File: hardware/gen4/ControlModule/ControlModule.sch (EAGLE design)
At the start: 16 parts, among them IC1 XMEGA16A4A

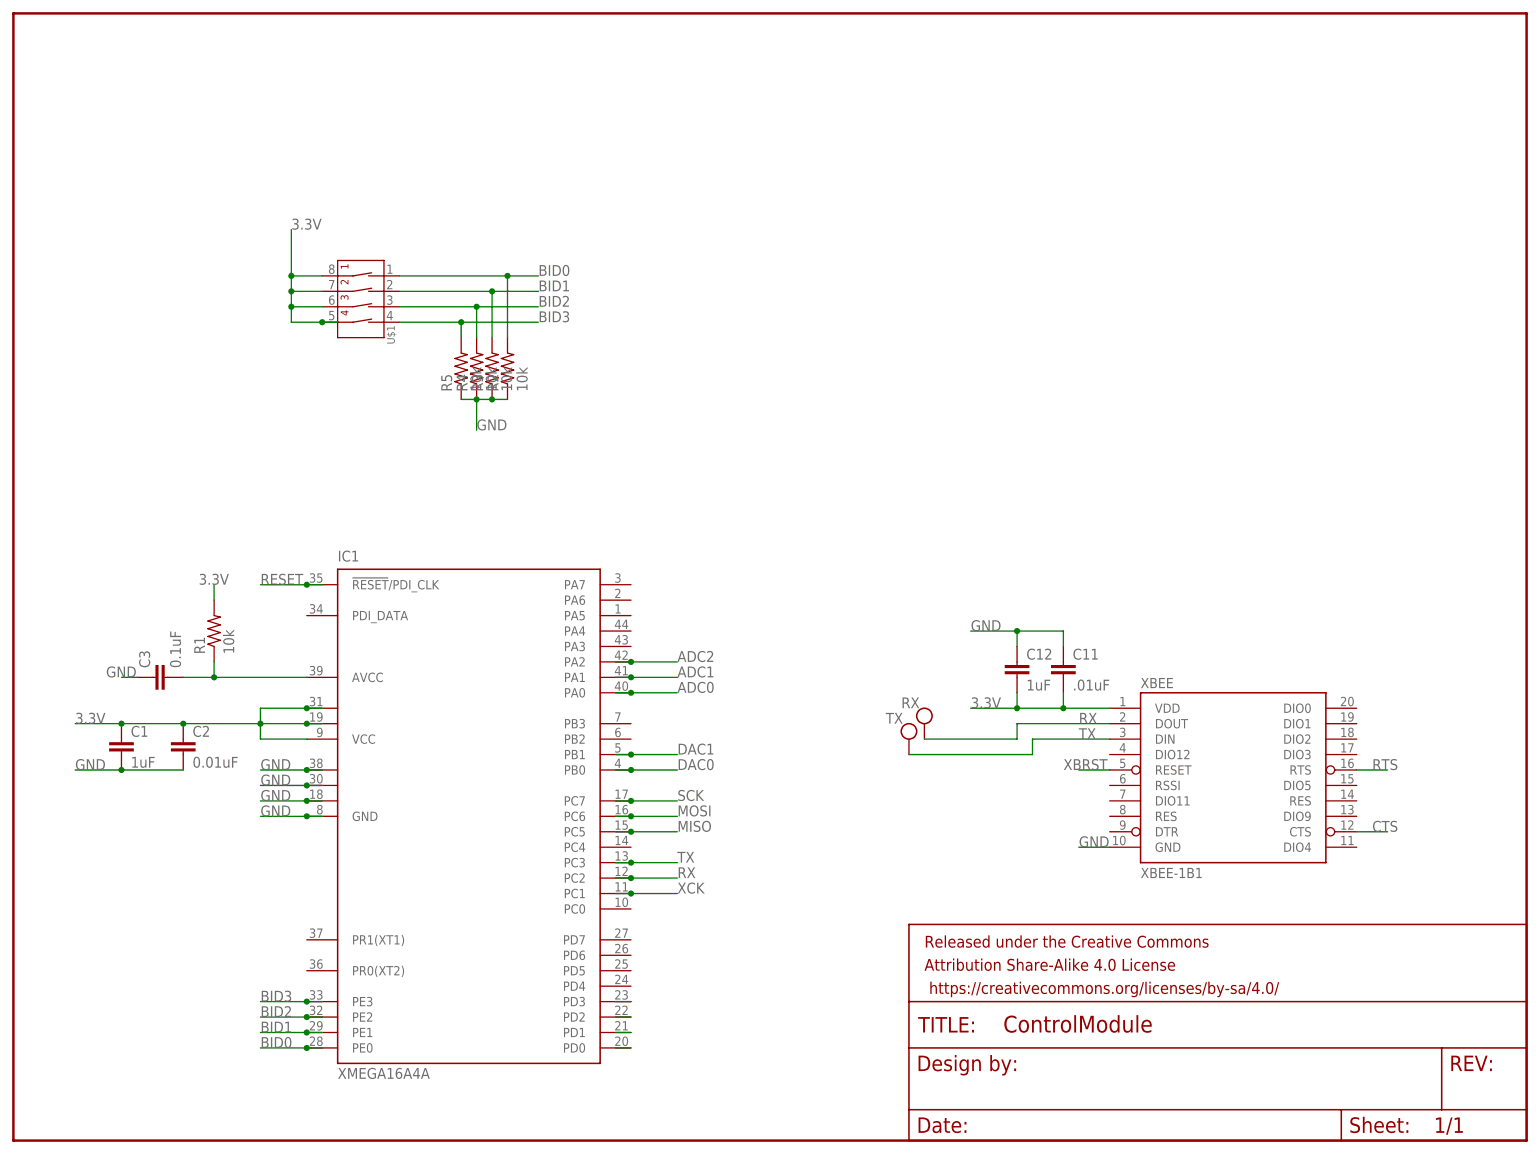
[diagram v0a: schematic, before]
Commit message: Working on xbee stuff for microboard
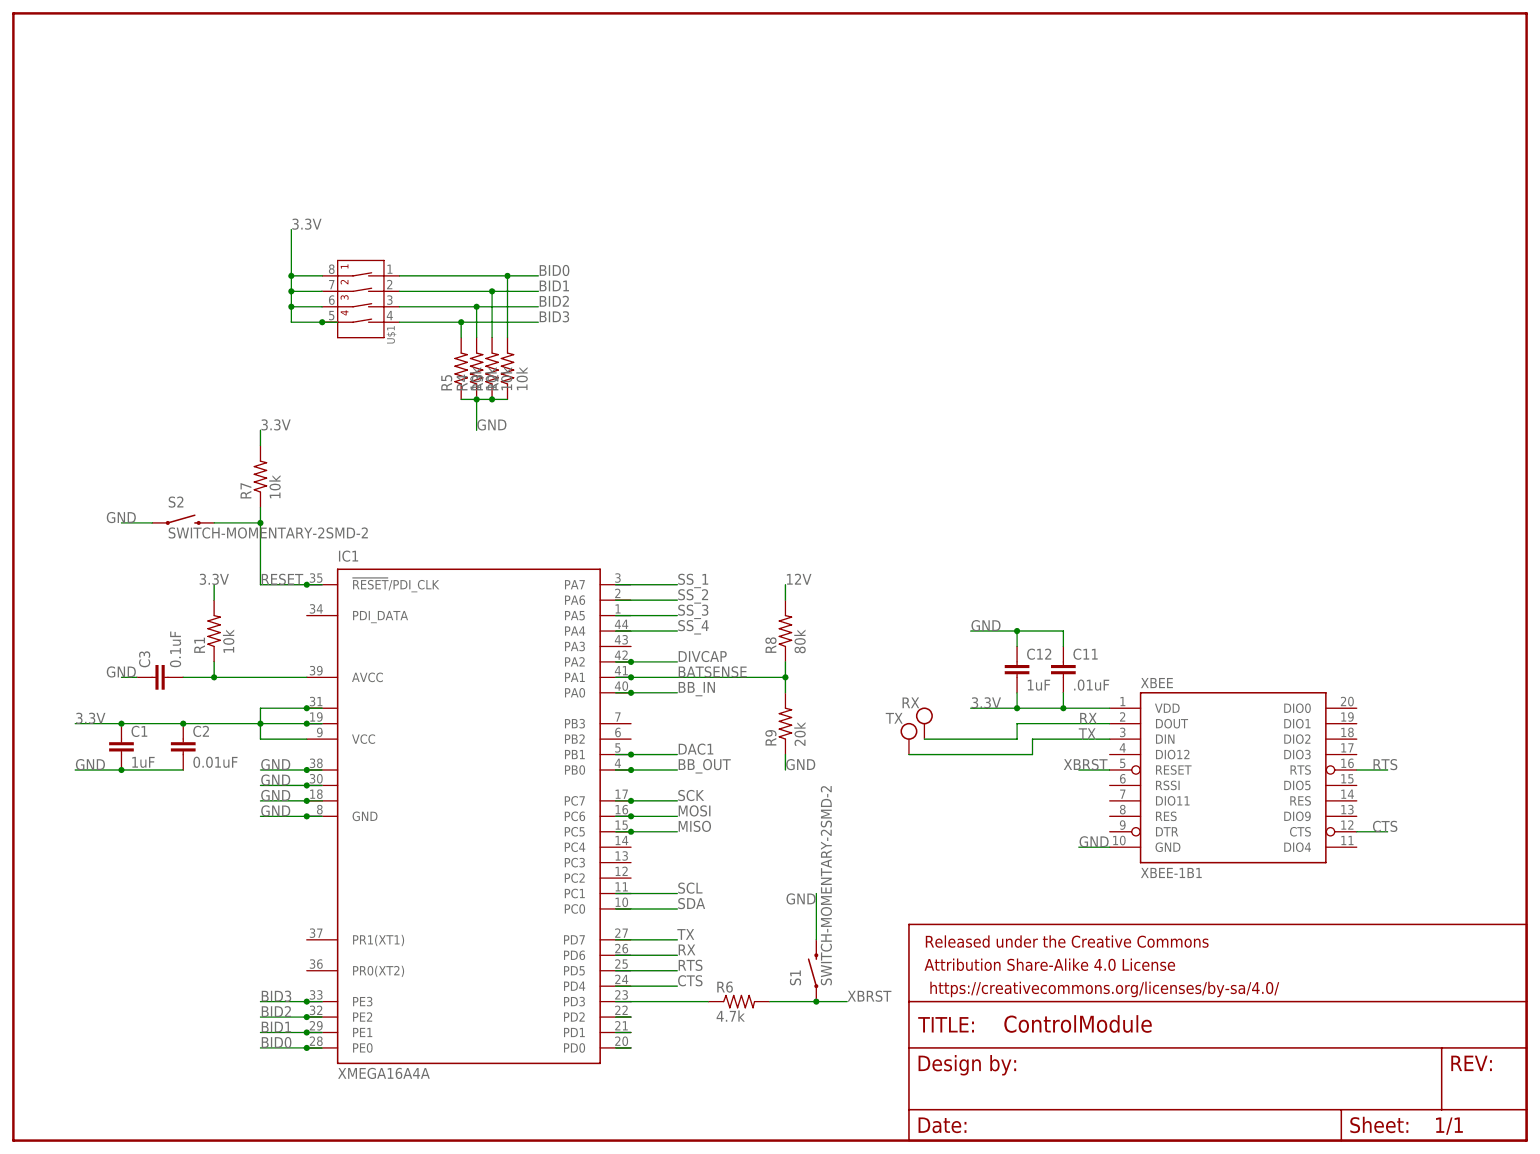
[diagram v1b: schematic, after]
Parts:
- added R6: 4.7k, SparkFun-Passives:RESISTOR0805-RES
- added R7: 10k, SparkFun-Passives:RESISTOR0805-RES
- added R8: 80k, SparkFun-Passives:RESISTOR0805-RES
- added R9: 20k, SparkFun-Passives:RESISTOR0805-RES
- added S1, S2: SWITCH-MOMENTARY-2SMD-2, SparkFun-Electromechanical:SWITCH-MOMENTARY-2SMD-2
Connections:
- net ADC0 renamed BB_IN
- net ADC2 renamed DIVCAP
- net DAC0 renamed BB_OUT
- removed net ADC1: IC1.PA1
- removed net XCK: IC1.PC1
- new net 12V: R8.2
- new net BATSENSE: IC1.PA1, R8.1, R9.2
- net 3.3V: now also R7.2
- net GND: now also R9.1, S1.2, S2.1
- net N$5: now also R6.1
- net RESET: now also R7.1, S2.2
- net RX: no longer IC1.PC2
- net TX: no longer IC1.PC3
- net XBRST: now also R6.2, S1.1
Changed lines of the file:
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@@
 <part name="RX" library="gen3" deviceset="TEST_PT" device=""/>
 <part name="TX" library="gen3" deviceset="TEST_PT" device=""/>
+<part name="R6" library="SparkFun-Passives" deviceset="RESISTOR" device="0805-RES" value="4.7k"/>
+<part name="S1" library="SparkFun-Electromechanical" deviceset="SWITCH-MOMENTARY-2" device="SMD-2"/>
+<part name="S2" library="SparkFun-Electromechanical" deviceset="SWITCH-MOMENTARY-2" device="SMD-2"/>
+<part name="R7" library="SparkFun-Passives" deviceset="RESISTOR" device="0805-RES" value="10k"/>
+<part name="R8" library="SparkFun-Passives" deviceset="RESISTOR" device="0805-RES" value="80k"/>
+<part name="R9" library="SparkFun-Passives" deviceset="RESISTOR" device="0805-RES" value="20k"/>
 </parts>
 <sheets>
@@
 <instance part="RX" gate="G$1" x="149.86" y="68.58"/>
 <instance part="TX" gate="G$1" x="147.32" y="66.04"/>
+<instance part="R6" gate="G$1" x="119.38" y="22.86"/>
+<instance part="S1" gate="G$1" x="132.08" y="27.94" rot="R90"/>
+<instance part="S2" gate="G$1" x="27.94" y="101.6"/>
+<instance part="R7" gate="G$1" x="40.64" y="109.22" rot="R90"/>
+<instance part="R8" gate="G$1" x="127" y="83.82" rot="R90"/>
+<instance part="R9" gate="G$1" x="127" y="68.58" rot="R90"/>
 </instances>
 <busses>
@@
 </net>
 <net name="TX" class="0">
-<segment>
-<wire x1="99.06" y1="45.72" x2="101.6" y2="45.72" width="0.1524" layer="91"/>
-<label x="109.22" y="45.72" size="1.778" layer="95"/>
-<pinref part="IC1" gate="G$1" pin="PC3"/>
-<wire x1="101.6" y1="45.72" x2="109.22" y2="45.72" width="0.1524" layer="91"/>
-<junction x="101.6" y="45.72"/>
-</segment>
 <segment>
 <pinref part="XBEE" gate="G$1" pin="DIN"/>
@@
 <wire x1="167.64" y1="66.04" x2="180.34" y2="66.04" width="0.1524" layer="91"/>
 </segment>
+<segment>
+<wire x1="99.06" y1="33.02" x2="109.22" y2="33.02" width="0.1524" layer="91"/>
+<label x="109.22" y="33.02" size="1.778" layer="95"/>
+</segment>
 </net>
 <net name="RX" class="0">
-<segment>
-<wire x1="99.06" y1="43.18" x2="101.6" y2="43.18" width="0.1524" layer="91"/>
-<label x="109.22" y="43.18" size="1.778" layer="95"/>
-<pinref part="IC1" gate="G$1" pin="PC2"/>
-<wire x1="101.6" y1="43.18" x2="109.22" y2="43.18" width="0.1524" layer="91"/>
-<junction x="101.6" y="43.18"/>
-</segment>
 <segment>
 <pinref part="XBEE" gate="G$1" pin="DOUT"/>
@@
 <wire x1="165.1" y1="66.04" x2="149.86" y2="66.04" width="0.1524" layer="91"/>
 </segment>
-</net>
-<net name="XCK" class="0">
-<segment>
-<wire x1="99.06" y1="40.64" x2="101.6" y2="40.64" width="0.1524" layer="91"/>
-<label x="109.22" y="40.64" size="1.778" layer="95"/>
-<pinref part="IC1" gate="G$1" pin="PC1"/>
-<wire x1="101.6" y1="40.64" x2="109.22" y2="40.64" width="0.1524" layer="91"/>
-<junction x="101.6" y="40.64"/>
-</segment>
-</net>
-<net name="ADC0" class="0">
+<segment>
+<wire x1="99.06" y1="30.48" x2="109.22" y2="30.48" width="0.1524" layer="91"/>
+<label x="109.22" y="30.48" size="1.778" layer="95"/>
+</segment>
+</net>
+<net name="BB_IN" class="0">
 <segment>
 <wire x1="99.06" y1="73.66" x2="101.6" y2="73.66" width="0.1524" layer="91"/>
@@
 </segment>
 </net>
-<net name="ADC1" class="0">
+<net name="BATSENSE" class="0">
 <segment>
 <wire x1="99.06" y1="76.2" x2="101.6" y2="76.2" width="0.1524" layer="91"/>
 <label x="109.22" y="76.2" size="1.778" layer="95"/>
 <pinref part="IC1" gate="G$1" pin="PA1"/>
-<wire x1="101.6" y1="76.2" x2="109.22" y2="76.2" width="0.1524" layer="91"/>
 <junction x="101.6" y="76.2"/>
-</segment>
-</net>
-<net name="ADC2" class="0">
+<wire x1="101.6" y1="76.2" x2="127" y2="76.2" width="0.1524" layer="91"/>
+<wire x1="127" y1="76.2" x2="127" y2="73.66" width="0.1524" layer="91"/>
+<wire x1="127" y1="76.2" x2="127" y2="78.74" width="0.1524" layer="91"/>
+<junction x="127" y="76.2"/>
+<pinref part="R8" gate="G$1" pin="1"/>
+<pinref part="R9" gate="G$1" pin="2"/>
+</segment>
+</net>
+<net name="DIVCAP" class="0">
 <segment>
 <wire x1="99.06" y1="78.74" x2="101.6" y2="78.74" width="0.1524" layer="91"/>
@@
 <wire x1="48.26" y1="91.44" x2="40.64" y2="91.44" width="0.1524" layer="91"/>
 <junction x="48.26" y="91.44"/>
+<wire x1="40.64" y1="91.44" x2="40.64" y2="101.6" width="0.1524" layer="91"/>
+<wire x1="40.64" y1="101.6" x2="40.64" y2="104.14" width="0.1524" layer="91"/>
+<wire x1="40.64" y1="101.6" x2="33.02" y2="101.6" width="0.1524" layer="91"/>
+<junction x="40.64" y="101.6"/>
+<pinref part="S2" gate="G$1" pin="2"/>
+<pinref part="R7" gate="G$1" pin="1"/>
 </segment>
 </net>
@@
 <junction x="165.1" y="83.82"/>
 <label x="157.48" y="83.82" size="1.778" layer="95"/>
+</segment>
+<segment>
+<pinref part="S1" gate="G$1" pin="2"/>
+<wire x1="132.08" y1="33.02" x2="132.08" y2="40.64" width="0.1524" layer="91"/>
+<label x="132.08" y="40.64" size="1.778" layer="95" rot="R180"/>
+</segment>
+<segment>
+<pinref part="S2" gate="G$1" pin="1"/>
+<wire x1="22.86" y1="101.6" x2="17.78" y2="101.6" width="0.1524" layer="91"/>
+<label x="15.24" y="101.6" size="1.778" layer="95"/>
+</segment>
+<segment>
+<pinref part="R9" gate="G$1" pin="1"/>
+<wire x1="127" y1="63.5" x2="127" y2="60.96" width="0.1524" layer="91"/>
+<label x="127" y="60.96" size="1.778" layer="95"/>
 </segment>
 </net>
@@
 <junction x="172.72" y="71.12"/>
 </segment>
+<segment>
+<pinref part="R7" gate="G$1" pin="2"/>
+<wire x1="40.64" y1="114.3" x2="40.64" y2="116.84" width="0.1524" layer="91"/>
+<label x="40.64" y="116.84" size="1.778" layer="95"/>
+</segment>
 </net>
 <net name="N$1" class="0">
@@
 <wire x1="99.06" y1="22.86" x2="101.6" y2="22.86" width="0.1524" layer="91"/>
 <pinref part="IC1" gate="G$1" pin="PD3"/>
+<pinref part="R6" gate="G$1" pin="1"/>
+<wire x1="114.3" y1="22.86" x2="101.6" y2="22.86" width="0.1524" layer="91"/>
 </segment>
 </net>
@@
 </segment>
 </net>
-<net name="DAC0" class="0">
+<net name="BB_OUT" class="0">
 <segment>
 <wire x1="99.06" y1="60.96" x2="101.6" y2="60.96" width="0.1524" layer="91"/>
@@
 <label x="223.52" y="60.96" size="1.778" layer="95"/>
 </segment>
+<segment>
+<wire x1="99.06" y1="27.94" x2="109.22" y2="27.94" width="0.1524" layer="91"/>
+<label x="109.22" y="27.94" size="1.778" layer="95"/>
+</segment>
 </net>
 <net name="CTS" class="0">
@@
 <label x="223.52" y="50.8" size="1.778" layer="95"/>
 </segment>
+<segment>
+<wire x1="99.06" y1="25.4" x2="109.22" y2="25.4" width="0.1524" layer="91"/>
+<label x="109.22" y="25.4" size="1.778" layer="95"/>
+</segment>
 </net>
 <net name="XBRST" class="0">
@@
 <label x="172.72" y="60.96" size="1.778" layer="95"/>
 </segment>
-</net>
+<segment>
+<pinref part="R6" gate="G$1" pin="2"/>
+<pinref part="S1" gate="G$1" pin="1"/>
+<wire x1="124.46" y1="22.86" x2="132.08" y2="22.86" width="0.1524" layer="91"/>
+<wire x1="132.08" y1="22.86" x2="137.16" y2="22.86" width="0.1524" layer="91"/>
+<junction x="132.08" y="22.86"/>
+<label x="137.16" y="22.86" size="1.778" layer="95"/>
+</segment>
+</net>
+<net name="SCL" class="0">
+<segment>
+<wire x1="99.06" y1="40.64" x2="109.22" y2="40.64" width="0.1524" layer="91"/>
+<label x="109.22" y="40.64" size="1.778" layer="95"/>
+</segment>
+</net>
+<net name="SDA" class="0">
+<segment>
+<wire x1="99.06" y1="38.1" x2="109.22" y2="38.1" width="0.1524" layer="91"/>
+<label x="109.22" y="38.1" size="1.778" layer="95"/>
+</segment>
+</net>
+<net name="12V" class="0">
+<segment>
+<pinref part="R8" gate="G$1" pin="2"/>
+<wire x1="127" y1="88.9" x2="127" y2="91.44" width="0.1524" layer="91"/>
+<label x="127" y="91.44" size="1.778" layer="95"/>
+</segment>
+</net>
+<net name="SS_1" class="0">
+<segment>
+<wire x1="99.06" y1="91.44" x2="109.22" y2="91.44" width="0.1524" layer="91"/>
+<label x="109.22" y="91.44" size="1.778" layer="95"/>
+</segment>
+</net>
+<net name="SS_2" class="0">
+<segment>
+<wire x1="99.06" y1="88.9" x2="109.22" y2="88.9" width="0.1524" layer="91"/>
+<label x="109.22" y="88.9" size="1.778" layer="95"/>
+</segment>
+</net>
+<net name="SS_3" class="0">
+<segment>
+<wire x1="99.06" y1="86.36" x2="109.22" y2="86.36" width="0.1524" layer="91"/>
+<label x="109.22" y="86.36" size="1.778" layer="95"/>
+</segment>
+</net>
+<net name="SS_4" class="0">
+<segment>
+<wire x1="99.06" y1="83.82" x2="109.22" y2="83.82" width="0.1524" layer="91"/>
+<label x="109.22" y="83.82" size="1.778" layer="95"/>
+</segment>
+</net>
